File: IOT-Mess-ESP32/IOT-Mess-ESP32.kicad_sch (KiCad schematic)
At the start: 28 parts, among them J1 Conn_01x19_Pin, J10 Jumper, J2 Conn_01x19_Pin, J3 Jumper_2, J4 Jumper_2, J5 Conn_01x06_Pin, J7 Jumper, J8 Jumper, J9 Jumper, SW10 SW_Push, SW11 SW_Push, U10 USB_C_Receptacle_USB2.0_16P, U2 ESP32-C6-MINI-1, U4 ESP32-S2-WROVER, U6 ME6211C33M5

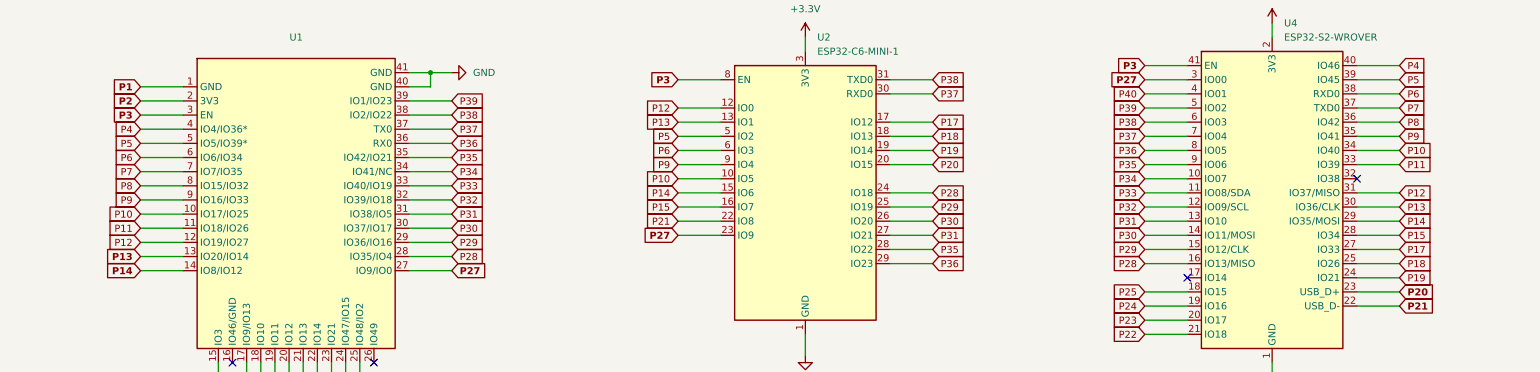
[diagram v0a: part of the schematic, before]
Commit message: did some works.
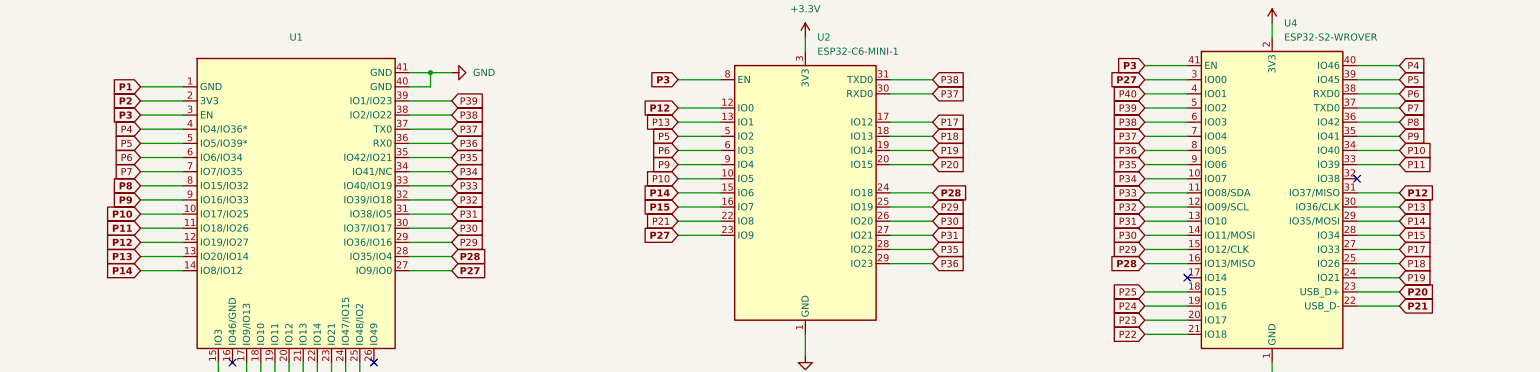
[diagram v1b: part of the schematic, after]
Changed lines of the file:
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@@
 			(font
 				(size 1.27 1.27)
+				(thickness 0.254)
+				(bold yes)
+				(color 255 0 255 1)
 			)
 			(justify left)
@@
 			(font
 				(size 1.27 1.27)
+				(thickness 0.254)
+				(bold yes)
+				(color 0 0 0 1)
 			)
 			(justify right)
@@
 			(font
 				(size 1.27 1.27)
+				(thickness 0.254)
+				(bold yes)
+				(color 255 0 255 1)
 			)
 			(justify right)
@@
 			(font
 				(size 1.27 1.27)
+				(thickness 0.254)
+				(bold yes)
+				(color 255 0 255 1)
 			)
 			(justify left)
@@
 			(font
 				(size 1.27 1.27)
+				(thickness 0.254)
+				(bold yes)
+				(color 255 0 255 1)
 			)
 			(justify right)
@@
 			(font
 				(size 1.27 1.27)
+				(thickness 0.254)
+				(bold yes)
+				(color 255 0 255 1)
 			)
 			(justify right)
@@
 			(font
 				(size 1.27 1.27)
+				(thickness 0.254)
+				(bold yes)
+				(color 0 0 0 1)
 			)
 			(justify right)
@@
 			(font
 				(size 1.27 1.27)
+				(thickness 0.254)
+				(bold yes)
+				(color 255 0 255 1)
 			)
 			(justify left)
@@
 			(font
 				(size 1.27 1.27)
+				(thickness 0.254)
+				(bold yes)
+				(color 0 0 0 1)
 			)
 			(justify right)
@@
 			(font
 				(size 1.27 1.27)
+				(thickness 0.254)
+				(bold yes)
+				(color 0 0 0 1)
 			)
 			(justify right)
@@
 			(font
 				(size 1.27 1.27)
+				(thickness 0.254)
+				(bold yes)
+				(color 0 0 0 1)
 			)
 			(justify right)
@@
 			(font
 				(size 1.27 1.27)
+				(thickness 0.254)
+				(bold yes)
+				(color 0 0 0 1)
 			)
 			(justify right)
